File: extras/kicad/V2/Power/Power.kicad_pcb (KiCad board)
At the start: 2 copper layers, 760.8 x 135.8 mm, 49 parts, among them J1 1X08_NO_SILK, J2 1X08_NO_SILK, J3 1X08_NO_SILK, J4 1X08_NO_SILK, J5 1X08, J6 1X08, J7 1X08, J8 1X08, SW1 SPDT-HIGH-AMP-SWITCHPTH, U1 CONN-TH_XT60, U1 TB6612FNG, U2 TB6612FNG, U8 POLULUMOTORBRACKETPPCB, X1 6, X2 6, X3 6, X4 6

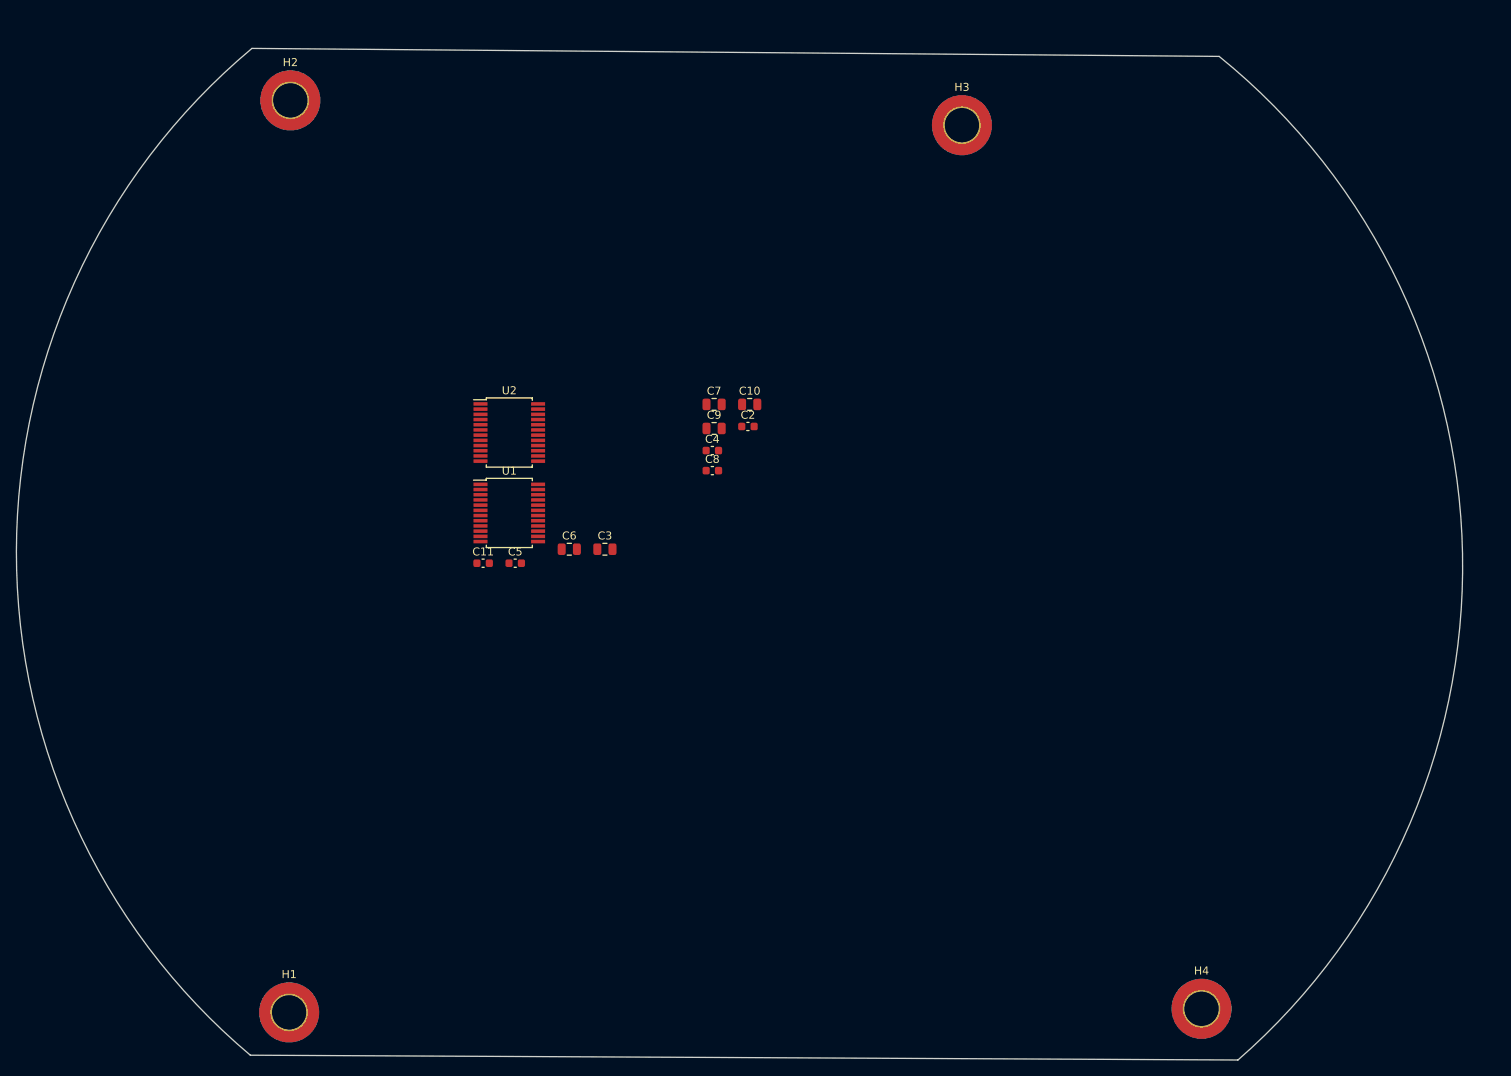
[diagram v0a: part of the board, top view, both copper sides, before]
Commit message: Add files via upload
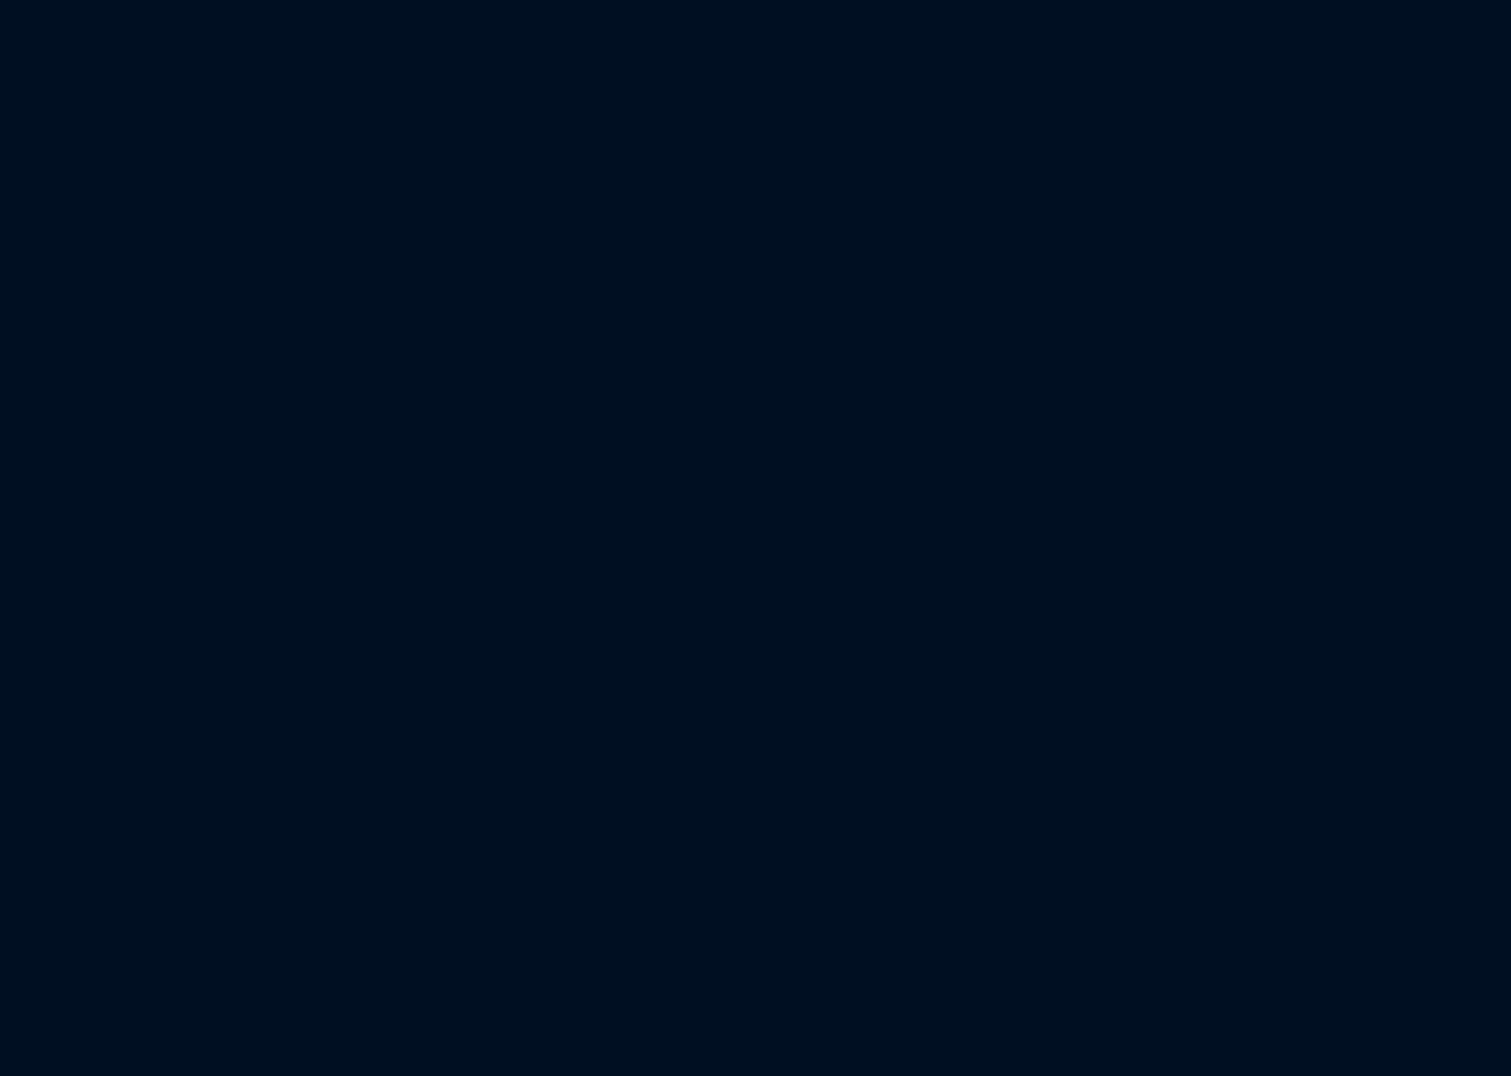
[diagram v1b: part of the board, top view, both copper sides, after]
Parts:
- removed C10, C3, C6, C7, C9: 22u, Capacitor_SMD:C_0805_2012Metric
- removed C11, C2, C4, C5, C8: 100n, Capacitor_SMD:C_0603_1608Metric
- removed H1, H2, H3, H4: Hole, MountingHole:MountingHole_4.3mm_M4_DIN965_Pad_TopBottom
- removed the U1 at (-141.6, 54.2)
- removed U2: TB6612FNG, Package_SO:SSOP-24_5.3x8.2mm_P0.65mm
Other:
- board size 760.8 x 135.8 mm -> 176 x 104.1 mm
- board text removed: "-"
- board text removed: "-1"
- board text removed: "-10"
- board text removed: "-11"
- board text removed: "-12"
- board text removed: "-14"
- board text removed: "-2"
- board text removed: "-3"
- board text removed: "-4"
- board text removed: "-5"
- board text removed: "-6"
- board text removed: "-7"
- board text removed: "-8"
- board text removed: "-9"
- board text removed: "1"
- board text removed: "10 Mbps"
- board text removed: "1751280"
- board text removed: "2"
- board text removed: "3"
- board text removed: "4"
- board text removed: "5"
- board text removed: "6"
- board text removed: "Artemis"
- board text removed: "ENC28J60-H"
- board text removed: "ESP32"
- board text removed: "Ethernet"
- board text removed: "FPGA"
- board text removed: "Featherwing"
- board text removed: "Grove"
- board text removed: "I2C"
- board text removed: "IMU"
- board text removed: "J1"
- board text removed: "J2"
- board text removed: "J3"
- board text removed: "J4"
- board text removed: "J5"
- board text removed: "J6"
- board text removed: "J7"
- board text removed: "J8"
- board text removed: "MS1"
- board text removed: "MicroMod"
- board text removed: "Mount holes for: Jetson Nano/ Beaglebone / Pi 4"
- board text removed: "Olimex.com"
- board text removed: "Optional"
- board text removed: "Qwiic"
- board text removed: "RP2040"
- board text removed: "SPI"
- board text removed: "STM32F405"
- board text removed: "SW1"
- board text removed: "Smartcar\nMotor board rev.0\ndesigned by Dimitris Platis\nhttp://plat.is/smartcar"
- board text removed: "Sparkfun.com"
- board text removed: "Teensy"
- board text removed: "U1"
- board text removed: "U4"
- board text removed: "U8"
- board text removed: "UEXT"
- board text removed: "USB-C"
- board text removed: "X1"
- board text removed: "X2"
- board text removed: "X3"
- board text removed: "X4"
- board text removed: "mikroe.com"
- board text removed: "nRF52840"
- board text removed: "pimoroni.com"
- board text removed: "seeed.cc"
